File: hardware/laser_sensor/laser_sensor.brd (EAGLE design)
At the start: 28.6 x 23.5 mm, 11 parts, among them IC1 NE555D, J1 B4B-XH-A(LF)(SN)

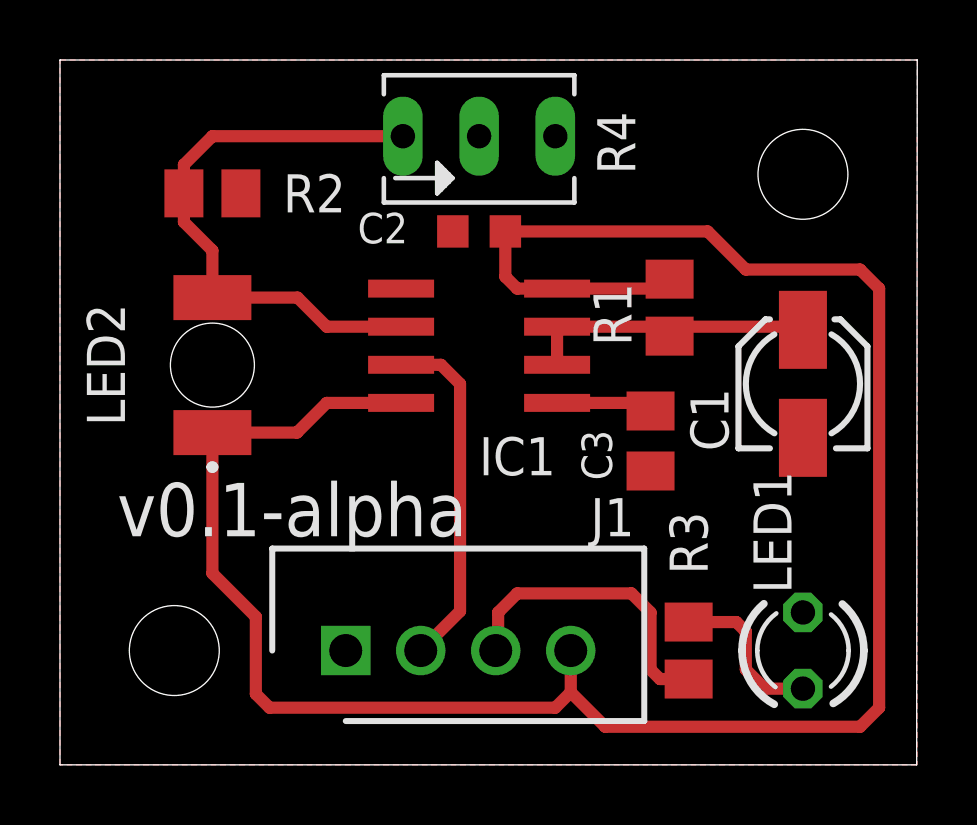
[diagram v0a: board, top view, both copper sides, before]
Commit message: sensor redesign
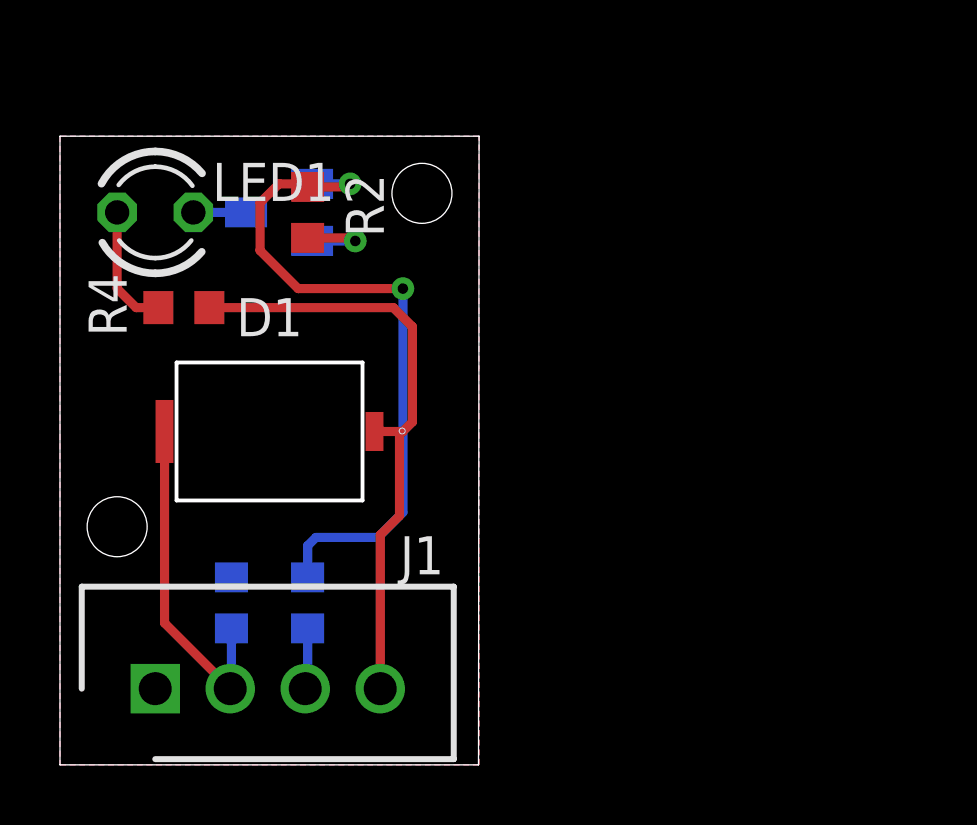
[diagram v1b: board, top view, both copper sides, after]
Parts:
- removed C1: 1u, rcl:153CLV-0405
- removed C2: 100n, rcl:C0603K
- removed C3: 10n, rcl:C0805K
- removed IC1: NE555D, linear:SO08
- removed LED2: SFH_2270_R, SFH_2270_R:SFH2270R
- added D1: SFH_2440_L, SFH_2440_L:SFH2440L
- added Q1: BC817-16LT1SMD, transistor-npn:SOT23-BEC
- R1: value 1M -> 100k; device resistor:M0805 -> rcl:R0603
- R2: value 15k -> 100k; device resistor:M0805 -> rcl:R0603
- R3: value 560 -> 10k; device resistor:M0805 -> rcl:R0603
- R4: value (none) -> 560; device pot:B64Y -> rcl:R0603
- moved LED1 26.1 mm to (3.17, 18.4), turned to 0 degrees
- moved R1 17.6 mm to (5.71, 5.40), flipped to the bottom
- moved R3 12.8 mm to (8.26, 5.40), flipped to the bottom
- moved R4 11.4 mm to (4.13, 15.2)
- moved J1 6.48 mm to (3.17, 2.54)
- moved R2 3.24 mm to (8.26, 18.4), turned to 270 degrees
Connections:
- net N$2 renamed LED
- removed net N$4: C3.1, IC1.5
- removed net N$5: LED1.A, R3.2
- new net N$2: LED1.K, Q1.C
- net +5V: now also D1.1, R4.2; no longer C2.1, IC1.4, IC1.8, LED2.1, R1.2
- net GND: now also Q1.E, R1.2, R2.2; no longer C1.-, C2.2, C3.2, IC1.1, LED1.K, R2.1, R4.A, R4.S
- net N$1: now also LED1.A, R4.1; no longer C1.+, IC1.6, IC1.7, R1.1
- net N$3: now also Q1.B, R2.1, R3.2; no longer IC1.2, LED2.2, R2.2, R4.E
- net OUT: now also D1.2, R1.1; no longer IC1.3
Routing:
- net +5V: track 74.0 -> 20.5 mm
- net LED: track 10.2 -> 2.04 mm
- net N$1: track 9.77 -> 4.18 mm
- net N$5: track 5.47 -> 0.00 mm
- net N$3: track 19.2 -> 23.8 mm, vias 0 -> 2
- net N$4: track 3.23 -> 0.00 mm
- net GND: track 0.00 -> 3.07 mm, vias 0 -> 1
- net N$2: track 0.00 -> 1.76 mm
- added copper zone on layer 16, net GND
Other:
- board size 28.6 x 23.5 mm -> 14 x 21 mm
- board text removed: "DO NOT TOUCH ===>"
- board text removed: "v0.1-alpha"
- board text removed: "λ:"
